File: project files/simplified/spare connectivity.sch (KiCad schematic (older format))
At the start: 4 parts, among them J6 Self, J7 Conn_01x04, J8 Conn_01x04, U3 STM32F103CBUx

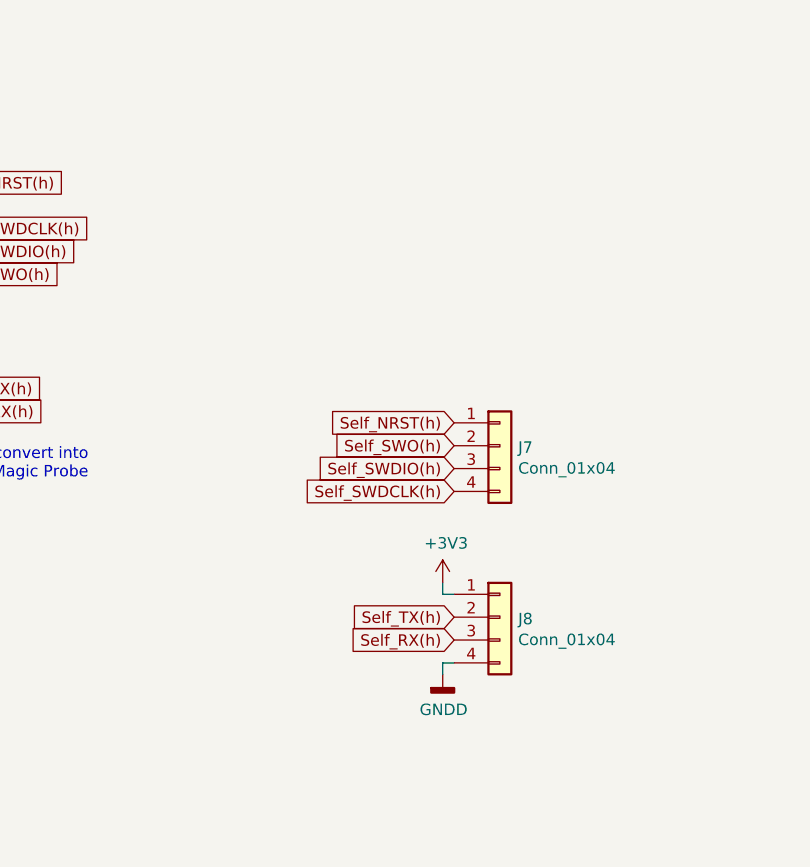
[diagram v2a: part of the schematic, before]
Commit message: STDC adapters
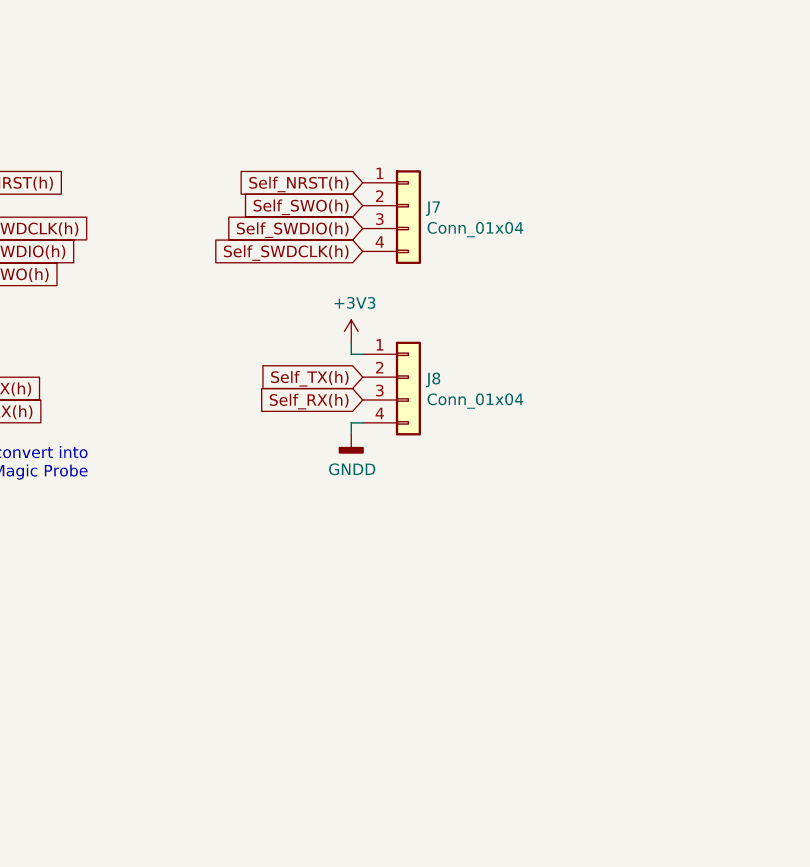
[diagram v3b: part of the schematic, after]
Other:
- moved on the sheet: J7, J8
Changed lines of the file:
@@
 L Connector_Generic:Conn_01x04 J7
 U 1 1 5FCDFBAC
-P 4200 2700
-F 0 "J7" H 4280 2692 50  0000 L CNN
-F 1 "Conn_01x04" H 4280 2601 50  0000 L CNN
-F 2 "Connector_PinHeader_2.54mm:PinHeader_1x04_P2.54mm_Vertical" H 4200 2700 50  0001 C CNN
-F 3 "~" H 4200 2700 50  0001 C CNN
-	1    4200 2700
+P 3800 1650
+F 0 "J7" H 3880 1642 50  0000 L CNN
+F 1 "Conn_01x04" H 3880 1551 50  0000 L CNN
+F 2 "Connector_PinHeader_2.54mm:PinHeader_1x04_P2.54mm_Vertical" H 3800 1650 50  0001 C CNN
+F 3 "~" H 3800 1650 50  0001 C CNN
+	1    3800 1650
 	1    0    0    -1
 $EndComp
@@
 L Connector_Generic:Conn_01x04 J8
 U 1 1 5FCE032D
-P 4200 3450
-F 0 "J8" H 4280 3442 50  0000 L CNN
-F 1 "Conn_01x04" H 4280 3351 50  0000 L CNN
-F 2 "Connector_PinHeader_2.54mm:PinHeader_1x04_P2.54mm_Vertical" H 4200 3450 50  0001 C CNN
-F 3 "~" H 4200 3450 50  0001 C CNN
-	1    4200 3450
+P 3800 2400
+F 0 "J8" H 3880 2392 50  0000 L CNN
+F 1 "Conn_01x04" H 3880 2301 50  0000 L CNN
+F 2 "Connector_PinHeader_2.54mm:PinHeader_1x04_P2.54mm_Vertical" H 3800 2400 50  0001 C CNN
+F 3 "~" H 3800 2400 50  0001 C CNN
+	1    3800 2400
 	1    0    0    -1
 $EndComp
-Text GLabel 4000 3450 0    50   Input ~ 0
+Text GLabel 3600 2400 0    50   Input ~ 0
 Self_TX(h)
-Text GLabel 4000 3550 0    50   Input ~ 0
+Text GLabel 3600 2500 0    50   Input ~ 0
 Self_RX(h)
 $Comp
 L power:GNDD #PWR054
 U 1 1 5FCE1122
-P 3950 3700
-F 0 "#PWR054" H 3950 3450 50  0001 C CNN
-F 1 "GNDD" H 3954 3545 50  0000 C CNN
-F 2 "" H 3950 3700 50  0001 C CNN
-F 3 "" H 3950 3700 50  0001 C CNN
-	1    3950 3700
+P 3550 2650
+F 0 "#PWR054" H 3550 2400 50  0001 C CNN
+F 1 "GNDD" H 3554 2495 50  0000 C CNN
+F 2 "" H 3550 2650 50  0001 C CNN
+F 3 "" H 3550 2650 50  0001 C CNN
+	1    3550 2650
 	1    0    0    -1
 $EndComp
@@
 L power:+3V3 #PWR053
 U 1 1 5FCE1839
-P 3950 3300
-F 0 "#PWR053" H 3950 3150 50  0001 C CNN
-F 1 "+3V3" H 3965 3473 50  0000 C CNN
-F 2 "" H 3950 3300 50  0001 C CNN
-F 3 "" H 3950 3300 50  0001 C CNN
-	1    3950 3300
+P 3550 2250
+F 0 "#PWR053" H 3550 2100 50  0001 C CNN
+F 1 "+3V3" H 3565 2423 50  0000 C CNN
+F 2 "" H 3550 2250 50  0001 C CNN
+F 3 "" H 3550 2250 50  0001 C CNN
+	1    3550 2250
 	1    0    0    -1
 $EndComp
 Wire Wire Line
-	4000 3350 3950 3350
+	3600 2300 3550 2300
 Wire Wire Line
-	3950 3350 3950 3300
+	3550 2300 3550 2250
 Wire Wire Line
-	4000 3650 3950 3650
+	3600 2600 3550 2600
 Wire Wire Line
-	3950 3650 3950 3700
-Text GLabel 4000 2700 0    50   Input ~ 0
+	3550 2600 3550 2650
+Text GLabel 3600 1650 0    50   Input ~ 0
 Self_SWO(h)
-Text GLabel 4000 2900 0    50   Input ~ 0
+Text GLabel 3600 1850 0    50   Input ~ 0
 Self_SWDCLK(h)
-Text GLabel 4000 2800 0    50   Input ~ 0
+Text GLabel 3600 1750 0    50   Input ~ 0
 Self_SWDIO(h)
-Text GLabel 4000 2600 0    50   Input ~ 0
+Text GLabel 3600 1550 0    50   Input ~ 0
 Self_NRST(h)
 $EndSCHEMATC
